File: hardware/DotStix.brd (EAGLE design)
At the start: 20.3 x 50 mm, 29 parts, among them IC2 SI1145, U1 ATMEGA328P-MU-QFN32, U2 TMP102, U4 9DoF IMU

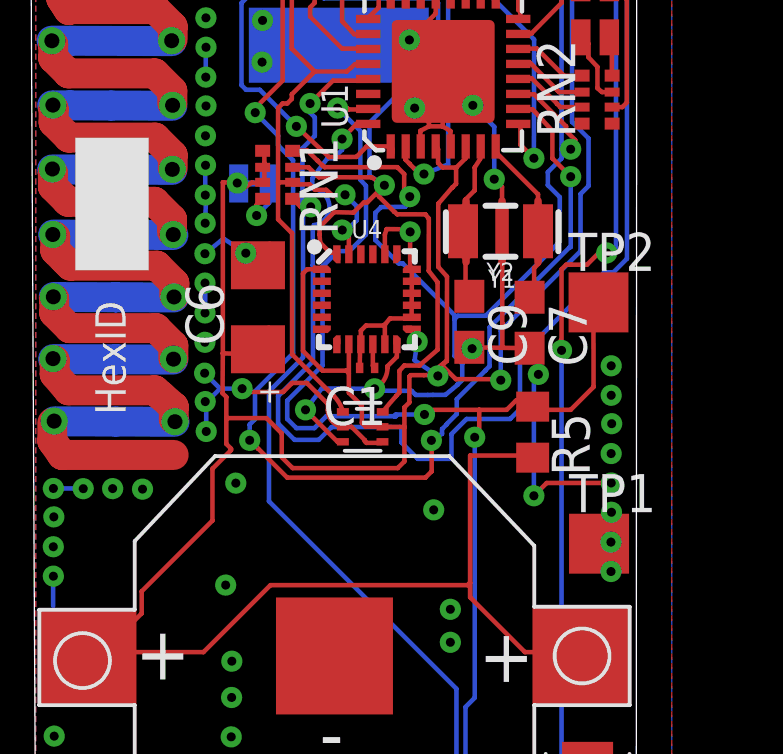
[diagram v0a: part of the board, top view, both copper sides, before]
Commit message: Add 9Dof: removed warnings
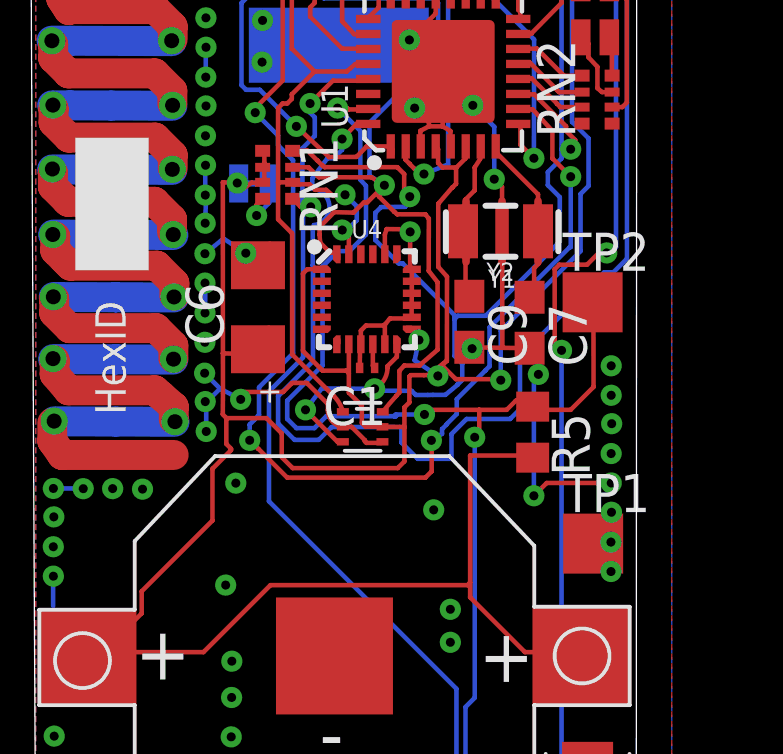
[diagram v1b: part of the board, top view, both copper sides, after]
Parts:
- moved TP2 0.20 mm to (18.6, 19.4)
- moved TP1 0.20 mm to (18.6, 11.4)
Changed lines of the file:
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@@
 <element name="U$2" library="adafruit" package="CR1220-SMD" value="" x="9.9568" y="7.6454" rot="R180"/>
 <element name="JP1" library="adafruit" package="1X06" value="" x="18.288" y="39.4208" rot="R270"/>
-<element name="TP1" library="testpad" package="TP20SQ" value="TPTP20SQ" x="18.77568125" y="11.38681875">
-<attribute name="TP_SIGNAL_NAME" value="" x="18.77568125" y="11.38681875" size="1.778" layer="27" display="off"/>
+<element name="TP1" library="testpad" package="TP20SQ" value="TPTP20SQ" x="18.580103125" y="11.389359375">
+<attribute name="TP_SIGNAL_NAME" value="" x="18.580103125" y="11.389359375" size="1.778" layer="27" display="off"/>
 </element>
-<element name="TP2" library="testpad" package="TP20SQ" value="TPTP20SQ" x="18.7579" y="19.431">
-<attribute name="TP_SIGNAL_NAME" value="" x="18.7579" y="19.431" size="1.778" layer="27" display="off"/>
+<element name="TP2" library="testpad" package="TP20SQ" value="TPTP20SQ" x="18.56231875" y="19.433540625">
+<attribute name="TP_SIGNAL_NAME" value="" x="18.56231875" y="19.433540625" size="1.778" layer="27" display="off"/>
 </element>
 <element name="D1" library="SparkFun" package="SOLARBIT-12X1" value="SOLAR-IXYS-" x="10.101578125" y="38.204140625" rot="MR270"/>
@@
 <wire x1="8.5471" y1="16.74621875" x2="8.244840625" y2="16.443959375" width="0.1524" layer="1"/>
 <wire x1="8.244840625" y1="16.443959375" x2="6.990078125" y2="16.443959375" width="0.1524" layer="1"/>
-<wire x1="6.990078125" y1="16.443959375" x2="6.87831875" y2="16.55571875" width="0.1524" layer="1"/>
-<via x="6.87831875" y="16.55571875" extent="1-16" drill="0.3"/>
-<wire x1="6.87831875" y1="16.55571875" x2="6.1442625" y2="16.55571875" width="0.1524" layer="16"/>
+<wire x1="6.990078125" y1="16.443959375" x2="6.830059375" y2="16.197578125" width="0.1524" layer="1"/>
+<via x="6.830059375" y="16.197578125" extent="1-16" drill="0.3"/>
+<wire x1="6.830059375" y1="16.197578125" x2="6.1442625" y2="16.55571875" width="0.1524" layer="16"/>
 <wire x1="6.1442625" y1="16.55571875" x2="5.628640625" y2="17.071340625" width="0.1524" layer="16"/>
 <wire x1="5.68198125" y1="16.12391875" x2="5.7124625" y2="16.12391875" width="0.1524" layer="16"/>
@@
 <wire x1="18.288" y1="37.1856" x2="18.288" y2="38.1508" width="0.1524" layer="1"/>
 <wire x1="19.6977" y1="35.7759" x2="18.288" y2="37.1856" width="0.1524" layer="1"/>
-<wire x1="17.526" y1="17.8308" x2="17.490440625" y2="18.150840625" width="0.1524" layer="1"/>
+<wire x1="17.526" y1="17.8308" x2="17.490440625" y2="18.150840625" width="0" layer="19" extent="1-16"/>
 <wire x1="17.526" y1="3.7109375" x2="17.526" y2="17.8308" width="0.1524" layer="16"/>
 <via x="9.144" y="26.0604" extent="1-16" drill="0.3"/>
@@
 <wire x1="18.3769" y1="20.6883" x2="17.846040625" y2="20.6883" width="0.1524" layer="1"/>
 <wire x1="17.846040625" y1="20.6883" x2="17.8435" y2="20.685759375" width="0.1524" layer="1"/>
-<wire x1="17.8435" y1="20.685759375" x2="17.6784" y2="20.685759375" width="0.1524" layer="1"/>
-<wire x1="17.6784" y1="20.685759375" x2="17.526" y2="20.533359375" width="0.1524" layer="1"/>
-<wire x1="17.526" y1="20.533359375" x2="17.526" y2="17.8308" width="0.1524" layer="1"/>
 <wire x1="7.7724" y1="16.4592" x2="8.91031875" y2="17.59711875" width="0.1524" layer="16"/>
 <wire x1="8.91031875" y1="17.59711875" x2="8.91031875" y2="22.34691875" width="0.1524" layer="16"/>
@@
 <wire x1="8.887459375" y1="24.56688125" x2="8.887459375" y2="22.616159375" width="0.1524" layer="16"/>
 <wire x1="8.887459375" y1="22.616159375" x2="9.16431875" y2="22.616159375" width="0.1524" layer="16"/>
+<wire x1="17.8435" y1="20.685759375" x2="17.447259375" y2="20.685759375" width="0.1524" layer="1"/>
+<wire x1="17.447259375" y1="20.685759375" x2="17.2974" y2="20.5359" width="0.1524" layer="1"/>
+<wire x1="17.2974" y1="20.5359" x2="17.2974" y2="18.0594" width="0.1524" layer="1"/>
+<wire x1="17.2974" y1="18.0594" x2="17.526" y2="17.8308" width="0.1524" layer="1"/>
 </signal>
 <signal name="RSEL">
@@
 <via x="17.8308" y="23.622" extent="1-16" drill="0.3"/>
 <via x="7.3152" y="25.7556" extent="1-16" drill="0.3"/>
-<wire x1="7.30758125" y1="16.46428125" x2="7.30758125" y2="15.53718125" width="0.1524" layer="16"/>
 <wire x1="17.8308" y1="21.2725" x2="17.8308" y2="23.622" width="0.1524" layer="16"/>
 <wire x1="17.8308" y1="21.2725" x2="17.800321875" y2="21.2725" width="0.1524" layer="16"/>
@@
 <wire x1="8.0772" y1="24.665940625" x2="8.57758125" y2="24.165559375" width="0.1524" layer="16"/>
 <wire x1="8.57758125" y1="24.165559375" x2="8.57758125" y2="17.73428125" width="0.1524" layer="16"/>
-<wire x1="8.57758125" y1="17.73428125" x2="7.30758125" y2="16.46428125" width="0.1524" layer="16"/>
 <wire x1="13.7033" y1="15.3797" x2="13.7033" y2="15.367" width="0.1524" layer="16"/>
 <wire x1="13.7033" y1="15.367" x2="13.54328125" y2="15.20698125" width="0.1524" layer="16"/>
@@
 <wire x1="13.197840625" y1="13.79981875" x2="13.197840625" y2="14.8209" width="0.1524" layer="1"/>
 <wire x1="13.197840625" y1="14.8209" x2="13.18768125" y2="14.831059375" width="0.1524" layer="1"/>
+<wire x1="7.30758125" y1="15.53718125" x2="7.30758125" y2="15.547340625" width="0.1524" layer="16"/>
+<wire x1="7.30758125" y1="15.547340625" x2="7.4422" y2="15.681959375" width="0.1524" layer="16"/>
+<wire x1="7.4422" y1="15.681959375" x2="7.4422" y2="16.5989" width="0.1524" layer="16"/>
+<wire x1="7.4422" y1="16.5989" x2="8.57758125" y2="17.73428125" width="0.1524" layer="16"/>
 </signal>
 <signal name="RIRQ">
@@
 <contactref element="U4" pad="8"/>
 <wire x1="12.28851875" y1="15.930878125" x2="12.45361875" y2="16.095978125" width="0.1524" layer="1"/>
-<wire x1="6.2255375" y1="16.40331875" x2="6.2357" y2="17.731740625" width="0.1524" layer="1"/>
-<wire x1="6.2357" y1="17.731740625" x2="6.2357" y2="23.434040625" width="0.1524" layer="1"/>
+<wire x1="6.240778125" y1="16.40331875" x2="6.238240625" y2="17.731740625" width="0.1524" layer="1"/>
+<wire x1="6.238240625" y1="17.731740625" x2="6.2357" y2="23.434040625" width="0.1524" layer="1"/>
 <wire x1="6.2357" y1="23.434040625" x2="6.715759375" y2="23.408640625" width="0.1524" layer="1"/>
 <via x="6.715759375" y="23.408640625" extent="1-16" drill="0.3"/>
@@
 <wire x1="6.581140625" y1="23.41118125" x2="6.76401875" y2="23.395940625" width="0.1524" layer="16"/>
 <wire x1="7.62" y1="17.34058125" x2="7.25678125" y2="17.7038" width="0.1524" layer="1"/>
-<wire x1="7.25678125" y1="17.7038" x2="6.2357" y2="17.731740625" width="0.1524" layer="1"/>
+<wire x1="7.25678125" y1="17.7038" x2="6.238240625" y2="17.731740625" width="0.1524" layer="1"/>
 <wire x1="10.43630625" y1="18.035140625" x2="10.43630625" y2="17.069353125" width="0.1524" layer="1"/>
 <wire x1="12.58880625" y1="18.535140625" x2="12.70761875" y2="18.535140625" width="0.1524" layer="1"/>
-<wire x1="12.70761875" y1="18.535140625" x2="12.715240625" y2="18.1229" width="0.1524" layer="1"/>
-<via x="12.715240625" y="18.1229" extent="1-16" drill="0.3"/>
-<wire x1="12.715240625" y1="18.1229" x2="12.62888125" y2="17.498059375" width="0.1524" layer="16"/>
+<wire x1="12.70761875" y1="18.535140625" x2="12.7736625" y2="18.176240625" width="0.1524" layer="1"/>
+<via x="12.7736625" y="18.176240625" extent="1-16" drill="0.3"/>
+<wire x1="12.7736625" y1="18.176240625" x2="12.62888125" y2="17.498059375" width="0.1524" layer="16"/>
 <wire x1="12.62888125" y1="17.498059375" x2="13.40358125" y2="16.979896875" width="0.1524" layer="16"/>
 <via x="13.40358125" y="16.979896875" extent="1-16" drill="0.3"/>
@@
 <wire x1="6.51001875" y1="14.554203125" x2="6.352540625" y2="14.71168125" width="0.1524" layer="1"/>
 <wire x1="6.352540625" y1="14.71168125" x2="6.352540625" y2="15.572740625" width="0.1524" layer="1"/>
-<wire x1="6.352540625" y1="15.572740625" x2="6.352540625" y2="16.276315625" width="0.1524" layer="1"/>
-<wire x1="6.352540625" y1="16.276315625" x2="6.2255375" y2="16.40331875" width="0.1524" layer="1"/>
 <wire x1="7.69111875" y1="15.572740625" x2="6.352540625" y2="15.572740625" width="0.1524" layer="1"/>
 <wire x1="9.48380625" y1="20.535140625" x2="9.046721875" y2="20.535140625" width="0.1524" layer="1"/>
@@
 <wire x1="10.99311875" y1="15.288259375" x2="11.55151875" y2="15.288259375" width="0.1524" layer="1"/>
 <wire x1="11.55151875" y1="15.288259375" x2="11.5566" y2="15.283178125" width="0.1524" layer="1"/>
+<wire x1="6.240778125" y1="16.40331875" x2="6.23315625" y2="15.69974375" width="0.1524" layer="1"/>
+<wire x1="6.23315625" y1="15.69974375" x2="6.352540625" y2="15.572740625" width="0.1524" layer="1"/>
 <wire x1="6.76401875" y1="23.395940625" x2="6.939278125" y2="23.238459375" width="0" layer="19" extent="1-16"/>
 </signal>
@@
 <wire x1="18.5928" y1="16.6116" x2="18.590259375" y2="18.823940625" width="0.1524" layer="1"/>
 <wire x1="18.590259375" y1="18.823940625" x2="18.590259375" y2="19.431" width="0.1524" layer="1"/>
-<wire x1="18.590259375" y1="19.431" x2="18.7579" y2="19.431" width="0.1524" layer="1"/>
+<wire x1="18.590259375" y1="19.431" x2="18.56231875" y2="19.433540625" width="0.1524" layer="1"/>
 <wire x1="17.8308" y1="15.8496" x2="18.5928" y2="16.6116" width="0.1524" layer="1"/>
 <wire x1="16.6116" y1="15.8496" x2="17.8308" y2="15.8496" width="0.1524" layer="1"/>
